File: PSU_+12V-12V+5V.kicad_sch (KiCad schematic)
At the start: 41 parts, among them J1 Screw_Terminal_01x02, J2 Screw_Terminal_01x02, Q1 BC557, Q2 BC557, Q3 BC547, Q4 BC547, U1 LM317L, U2 LM317L

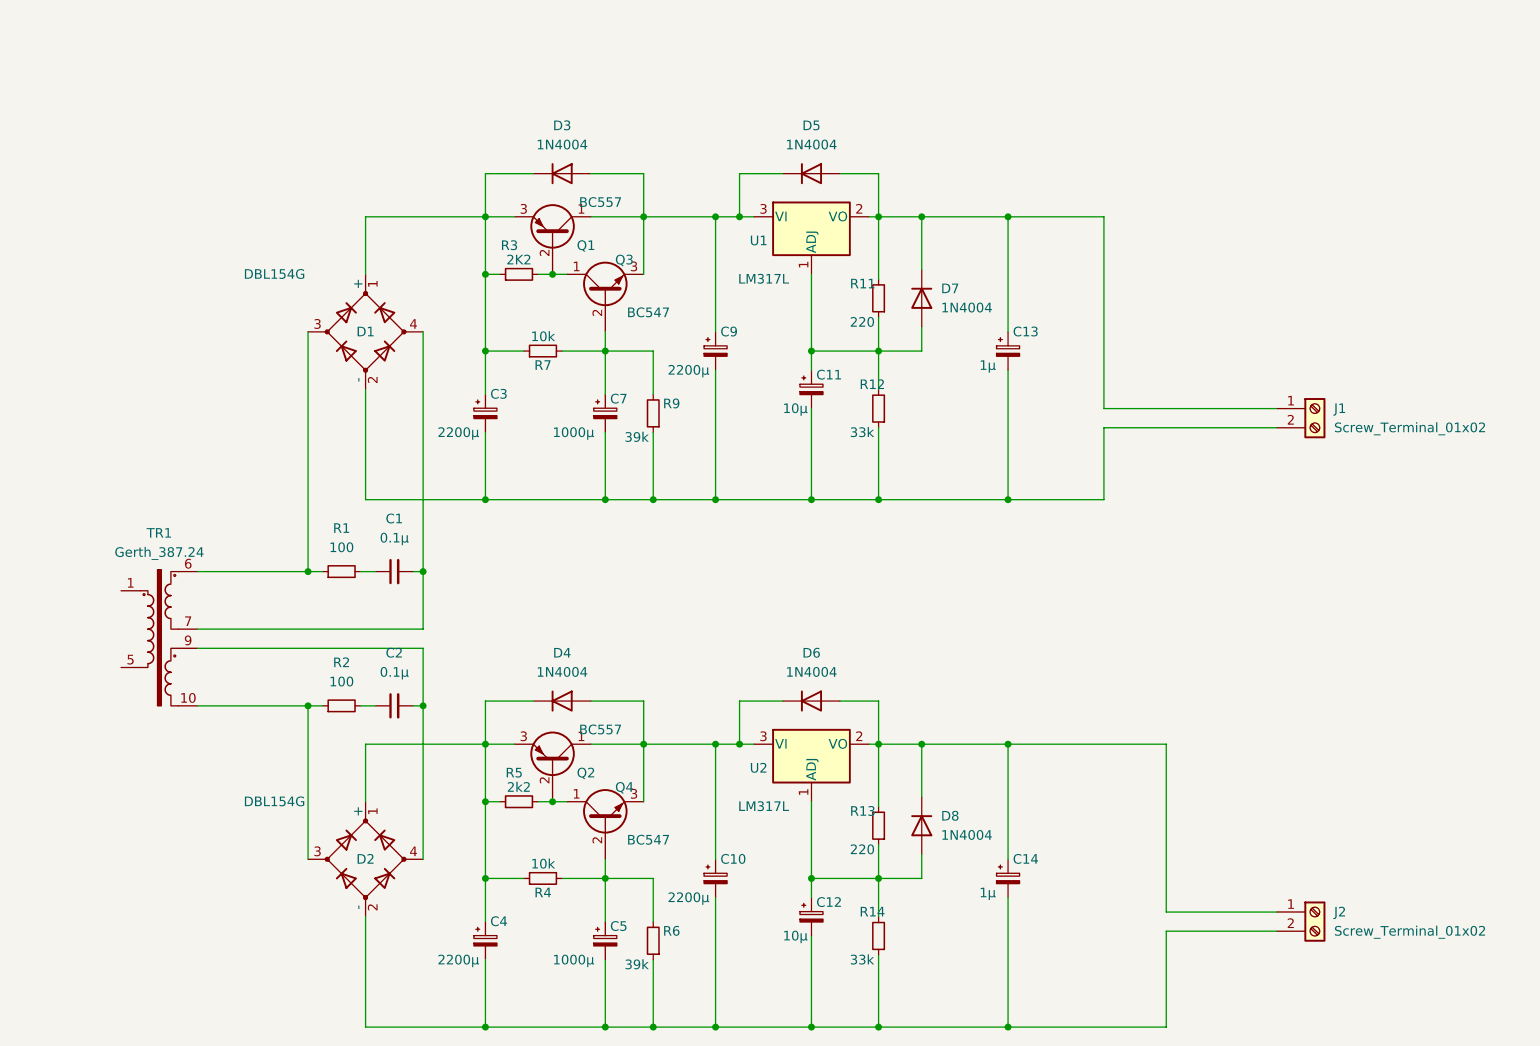
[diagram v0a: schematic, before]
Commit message: Some shifting
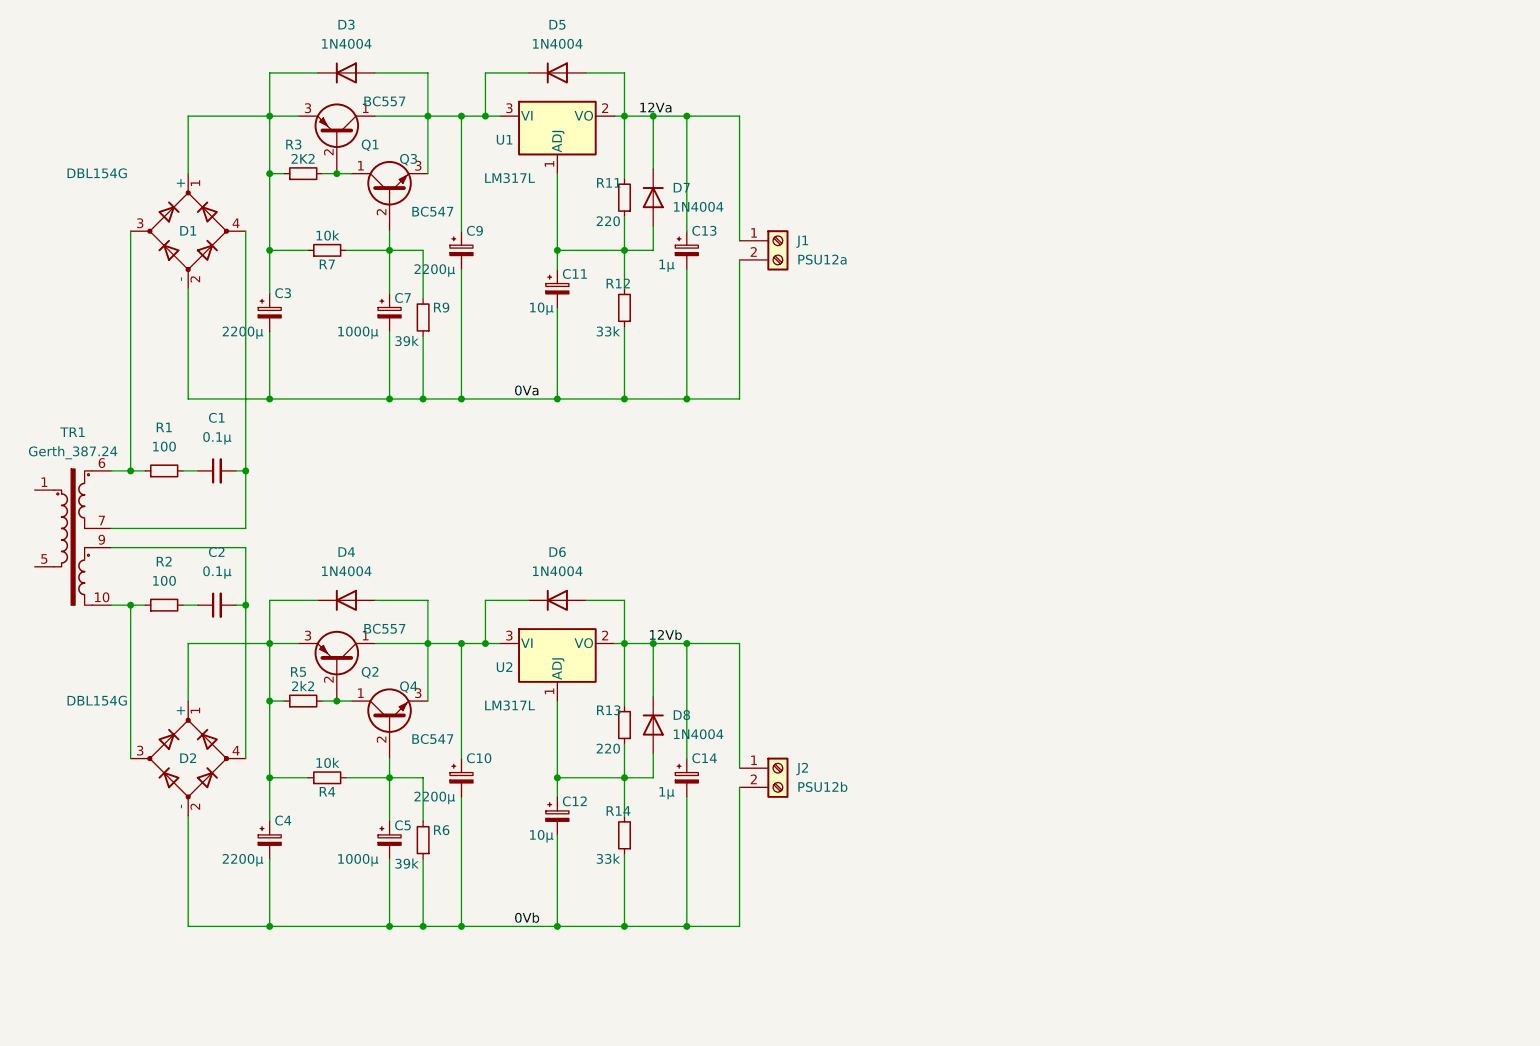
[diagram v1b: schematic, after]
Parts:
- J1: value Screw_Terminal_01x02 -> PSU12a
- J2: value Screw_Terminal_01x02 -> PSU12b
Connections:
- net 12Va: now reaches C13.1, D5.2 (A), D7.1 (K), J1.1 (Pin_1), R11.2, U1.2 (VO)
- net 0Va: now reaches C11.2, C13.2, C3.2, C7.2, C9.2, D1.2 (-), J1.2 (Pin_2), R12.1, R9.1
- net 0Vb: now reaches C10.2, C12.2, C14.2, C4.2, C5.2, D2.2 (-), J2.2 (Pin_2), R14.1, R6.1
- net 12Vb: now reaches C14.1, D6.2 (A), D8.1 (K), J2.1 (Pin_1), R13.2, U2.2 (VO)
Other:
- moved on the sheet: C1, C10, C11, C12, C13, C14, C2, C3, C4, C5, C7, C9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
